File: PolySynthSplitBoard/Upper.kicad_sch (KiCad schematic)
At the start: 17 parts, among them J801 A_UPPER, J802 B_UPPER, J803 C_UPPER, J804 D_UPPER, U801 CD40106BPWR, U802 CS5173

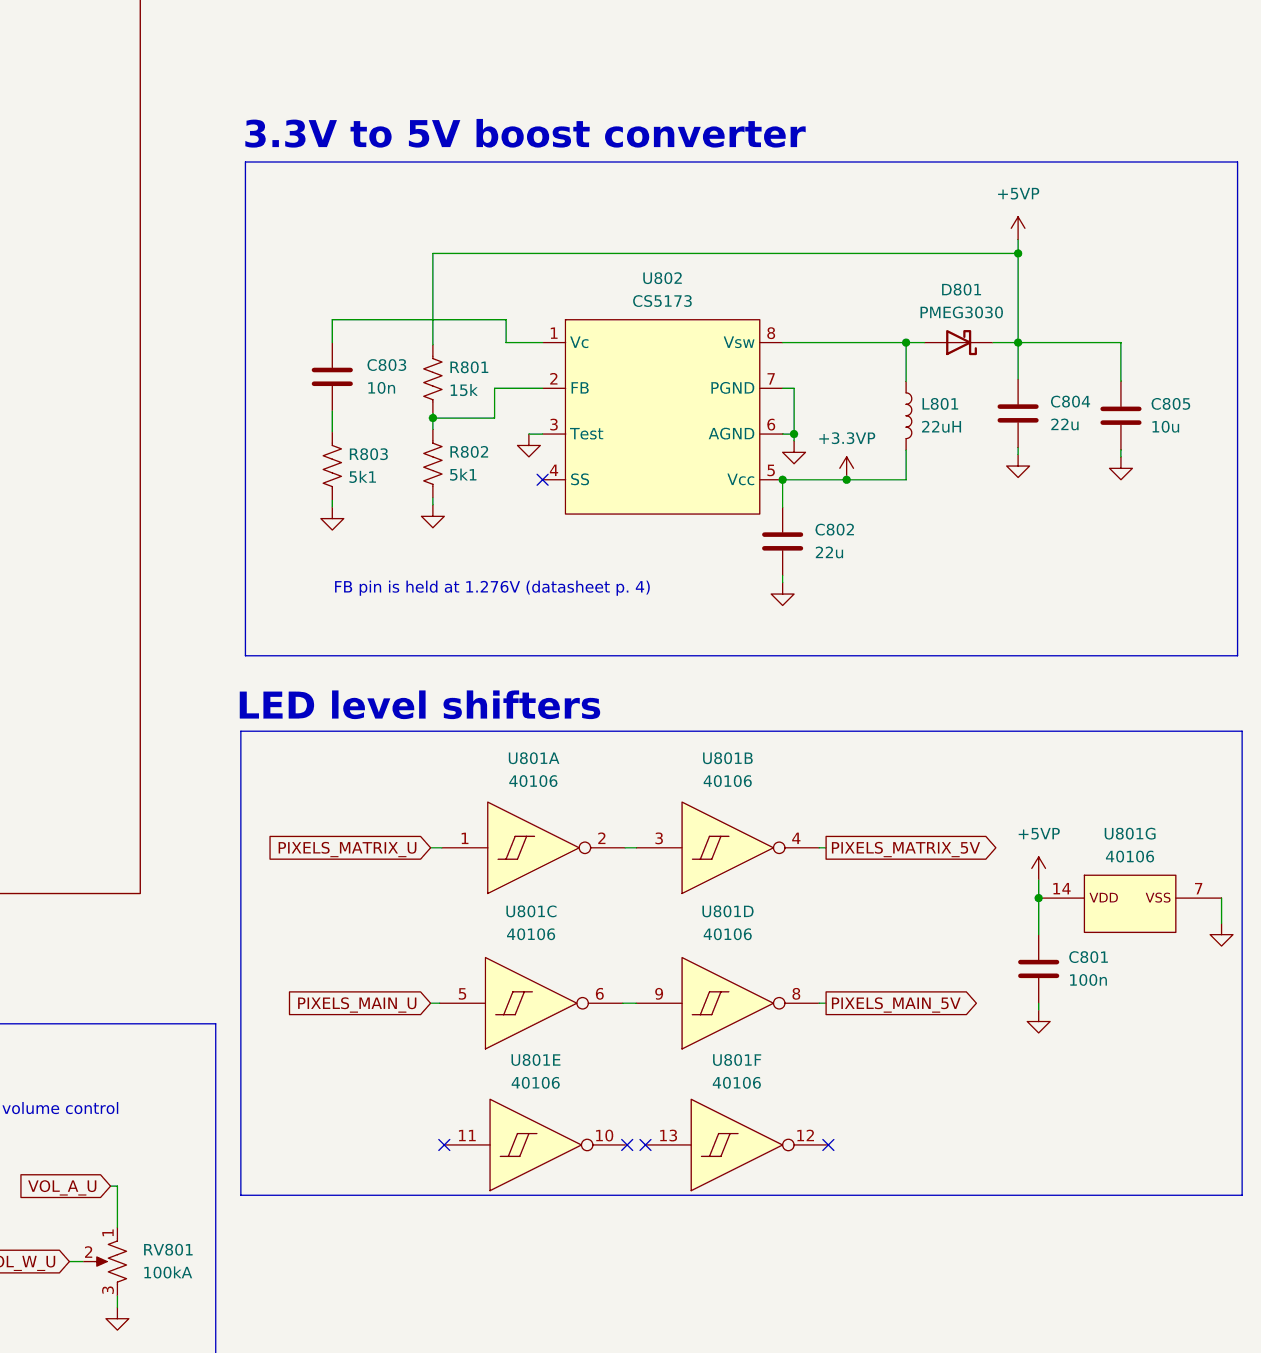
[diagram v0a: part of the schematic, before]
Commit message: motherboard rev2 passing DRC
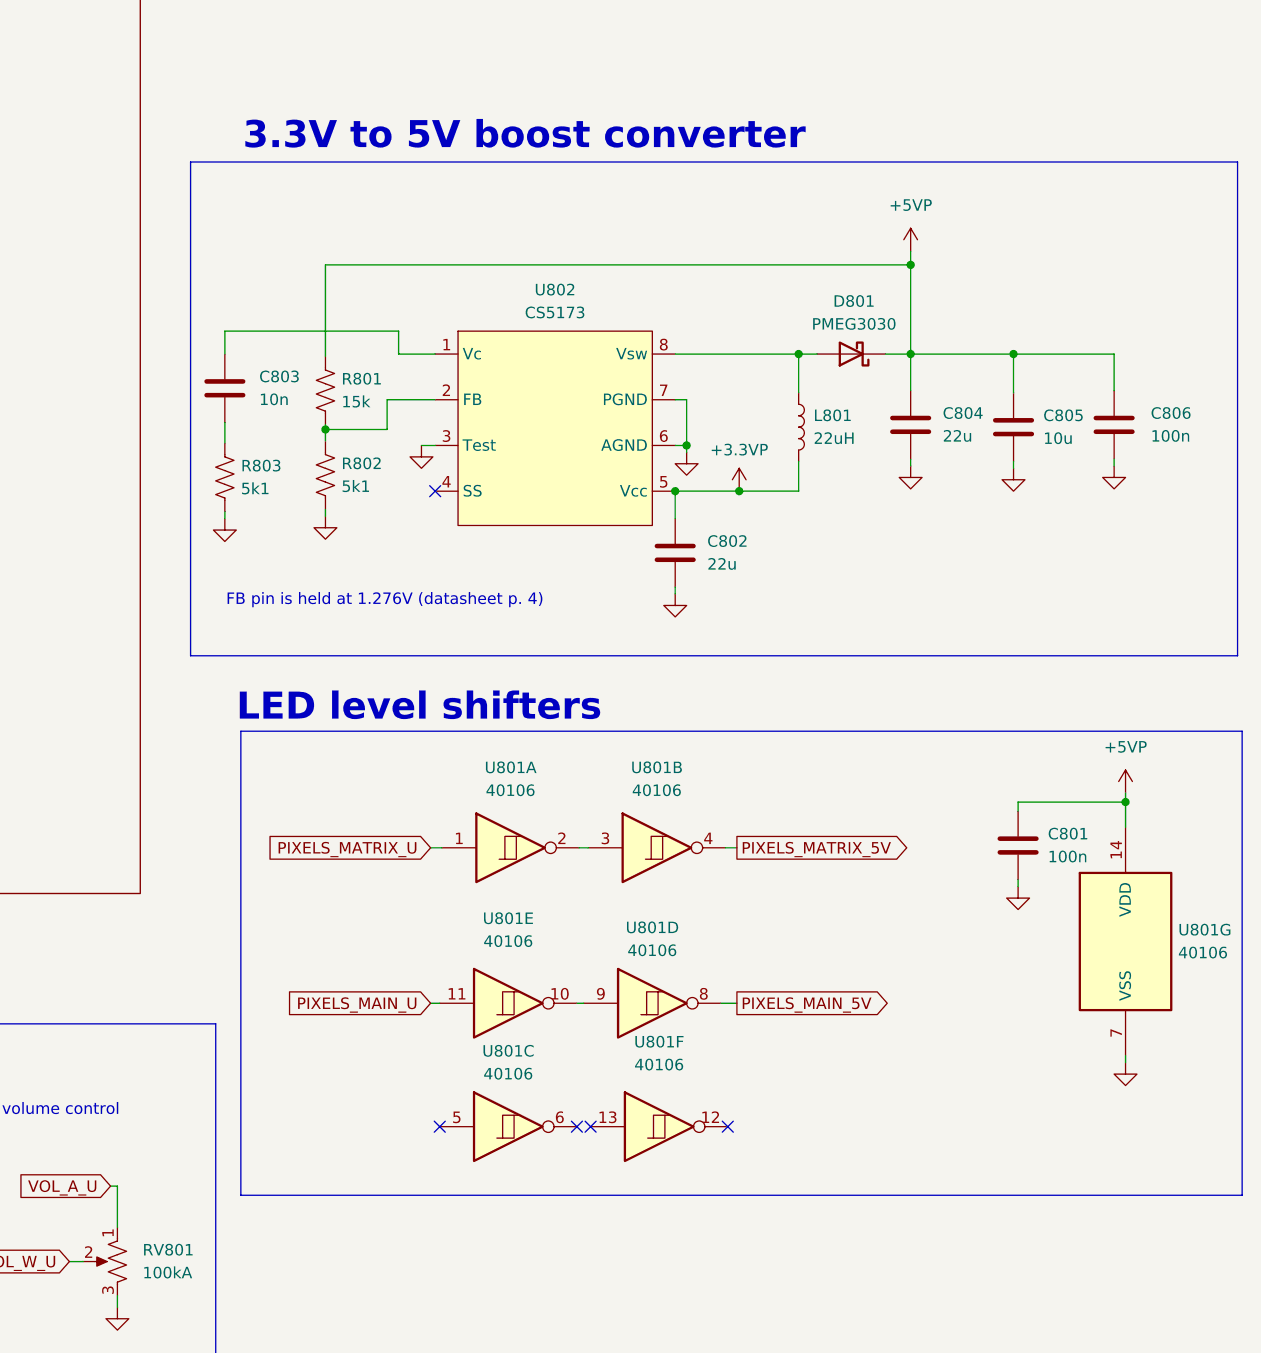
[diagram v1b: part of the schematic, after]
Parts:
- removed U801: CD40106BPWR, Package_SO:SOIC-14-16_3.9x9.9mm_P1.27mm, symbol PCM_4ms_IC:CD40106BPWR
- added C806: 100n, Capacitor_SMD:C_0805_2012Metric, symbol Device:C
- added U801: 40106, Package_SO:SOIC-14_3.9x8.7mm_P1.27mm, symbol 4xxx:40106
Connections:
- net +5VP: now also C806.1, U801.14 (VDD)
- net GNDA: now also C806.2, U801.7 (VSS)
- net PIXELS_MAIN_5V: now also U801.8
- net PIXELS_MAIN_U: now also U801.11
- net PIXELS_MATRIX_5V: now also U801.4
- net PIXELS_MATRIX_U: now also U801.1
- new net: U801.2, U801.3
- new net: U801.10, U801.9
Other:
- moved on the sheet: C802, C803, C804, C805, D801, L801, R801, R802, R803, U802
